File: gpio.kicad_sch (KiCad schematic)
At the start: 8 parts, among them J1 DF40C-100DP-0.4V(51), J2 DF40C-100DP-0.4V(51), J5 SerDes, U1 LFE5U-85F-6BG381C

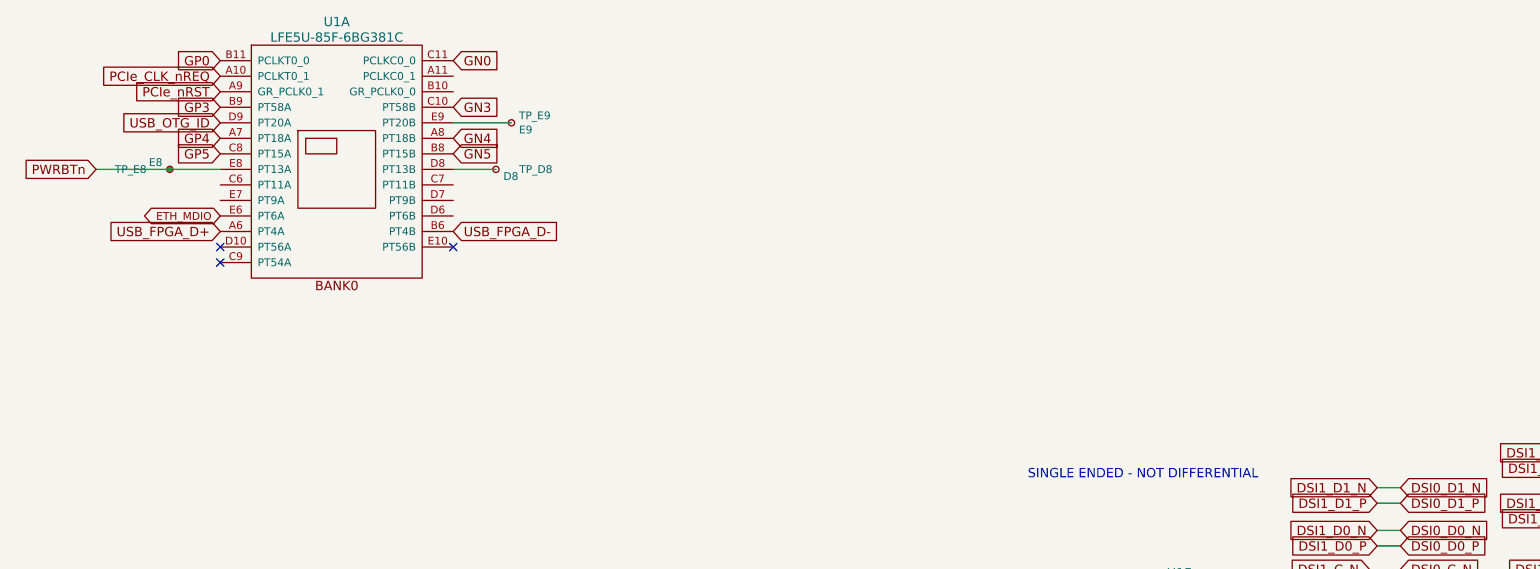
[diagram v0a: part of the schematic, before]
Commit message: Updating schematics
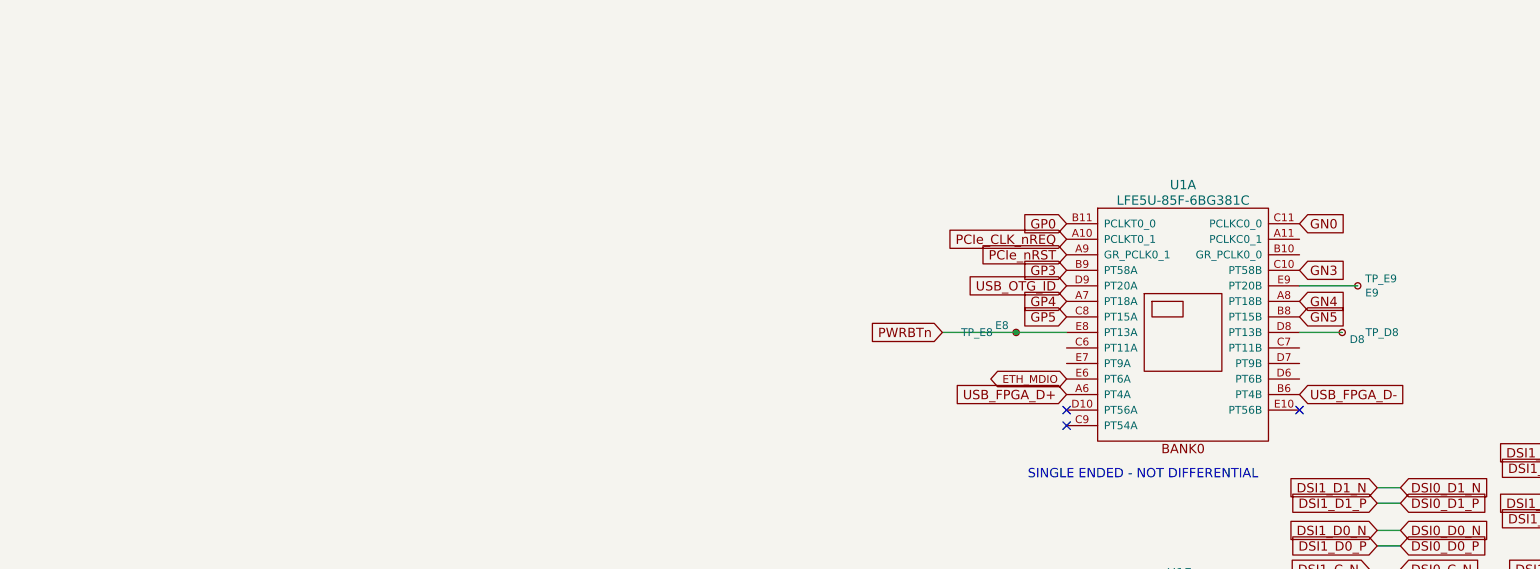
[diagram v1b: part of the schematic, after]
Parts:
- U1: Digike_y2 (none) -> 220-2071-ND; Digikey (none) -> 220-2177-ND; Koncar (none) -> FU004; LCSC (none) -> C446029; LowCost (none) -> 842-LFE5U12F6BG381C; MFG1 (none) -> Lattice; MFG2 (none) -> Lattice; MNF1_URL (none) -> www.latticesemi.com; MNF2_URL (none) -> www.latticesemi.com; MP_N2 (none) -> LFE5U-12F-6BG381C; Mouser (none) -> 842-LFE5U85F6BG381C; Mouser_URL (none) -> www.mouser.com; Side (none) -> T; price100_Mouse (none) -> 22.82$
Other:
- moved on the sheet: TP_D8, TP_E8, TP_E9, U1A
